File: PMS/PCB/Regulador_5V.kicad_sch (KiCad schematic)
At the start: 14 parts, among them U4 MP2303ADN

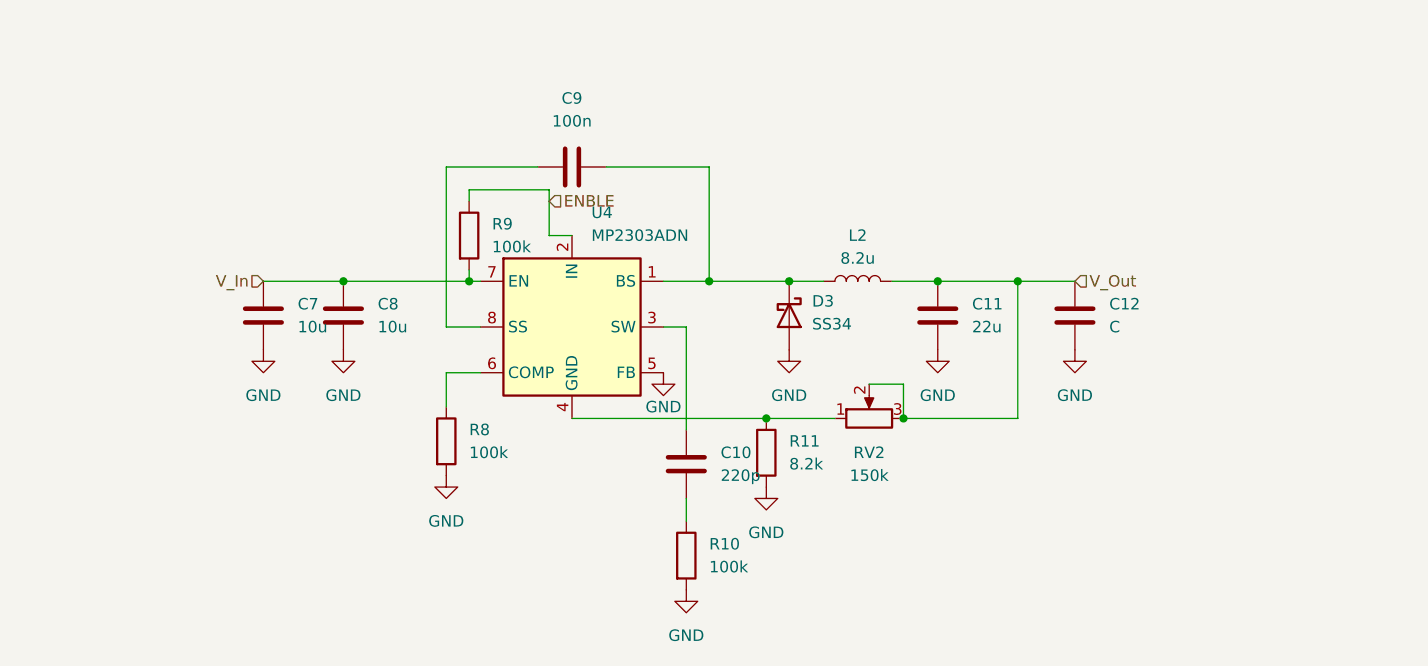
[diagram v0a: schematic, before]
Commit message: Continua Desarrollo
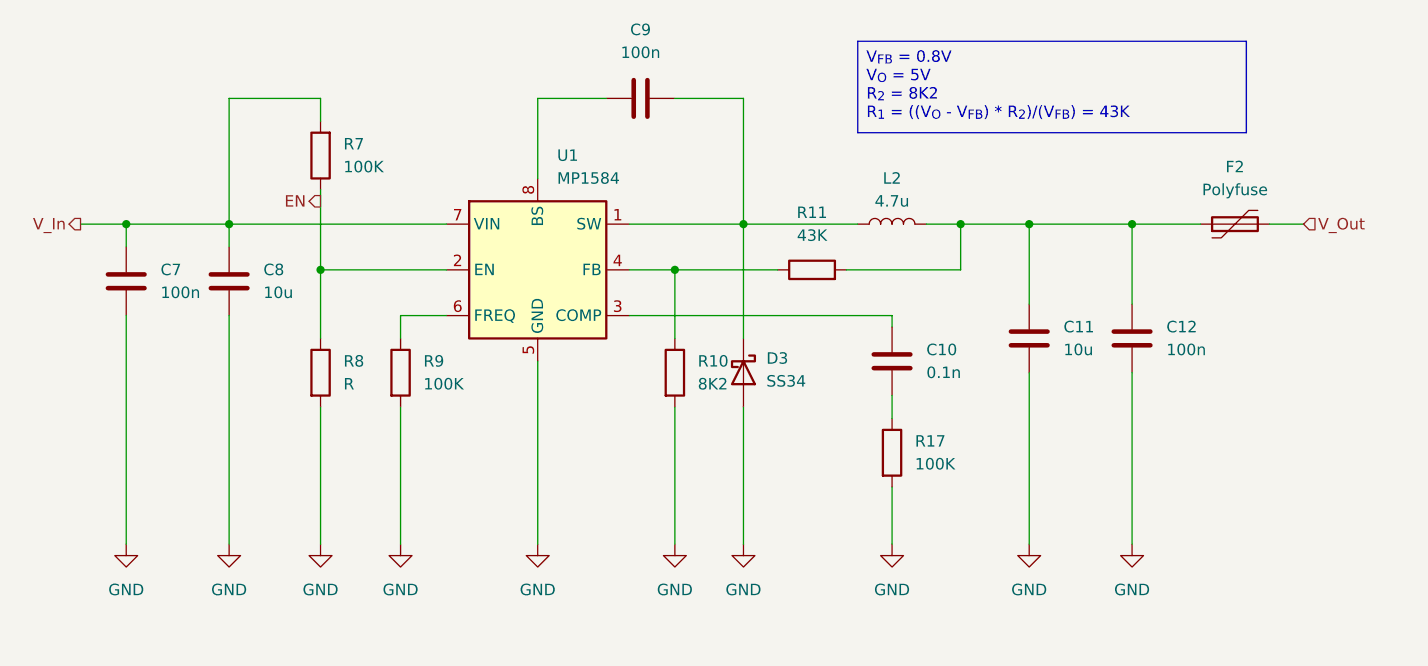
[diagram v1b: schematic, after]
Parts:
- removed D3: SS34, Diode_SMD:D_SMA, symbol Diode:SS34
- removed RV2: 150k, symbol Device:R_Potentiometer
- removed U4: MP2303ADN, Package_SO:SOIC-8-1EP_3.9x4.9mm_P1.27mm_EP2.62x3.51mm, symbol Regulator_Switching:MP2303ADN
- added D3: SS34, symbol Device:D_Schottky
- added F2: Polyfuse, symbol Device:Polyfuse
- added R17, R7: 100K, symbol Device:R
- added U1: MP1584, Package_SO:SOIC-8-1EP_3.9x4.9mm_P1.27mm_EP2.62x3.51mm, symbol CubeSat:MP1584EN
- C10: value 220p -> 0.1n
- C11: value 22u -> 10u
- C12: value C -> 100n
- C7: value 10u -> 100n
- L2: value 8.2u -> 4.7u
- R10: value 100k -> 8K2
- R11: value 8.2k -> 43K
- R8: value 100k -> R
- R9: value 100k -> 100K
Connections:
- net GND: now also R9.2, D3.2 (A), R17.2, U1.5 (GND); no longer R11.2
- net V_In: now also R7.2, U1.7 (VIN); no longer R9.2
- net V_Out: now also F2.2; no longer C11.1, C12.1, L2.2
- net at C9.2, L2.1: now also D3.1 (K), U1.1 (SW)
- net at C9.1: now also U1.8 (BS)
- net at R11.1: now also R10.1, U1.4 (FB)
- net at C10.2: now also R17.1; no longer R10.1
- net at C10.1: now also U1.3 (COMP)
- net EN: now reaches R8.1
- net EN: now also R7.1, U1.2 (EN)
- net ENBLE: no longer names the net of R9.1
- net ENBLE: now also U1.6 (FREQ)
- new net: C11.1, C12.1, F2.1, L2.2, R11.2
